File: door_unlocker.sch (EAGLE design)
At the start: 16 parts, among them IC1 LM2937, T1 2N3904

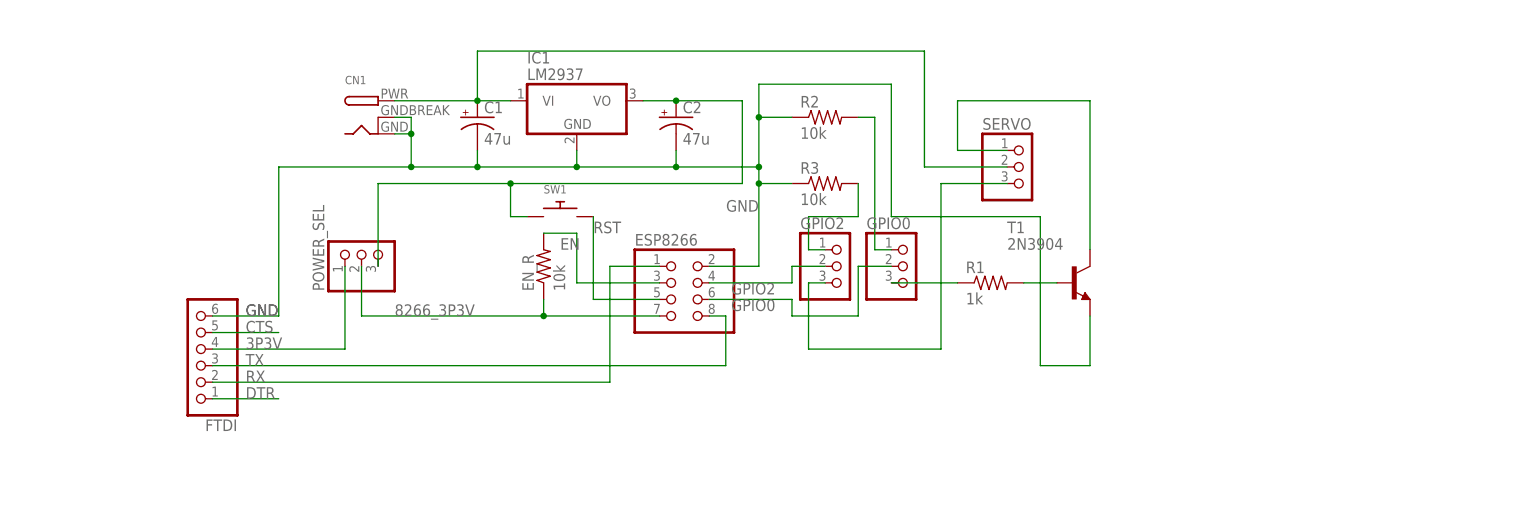
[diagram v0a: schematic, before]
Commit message: de-clusterfucked the schematic.
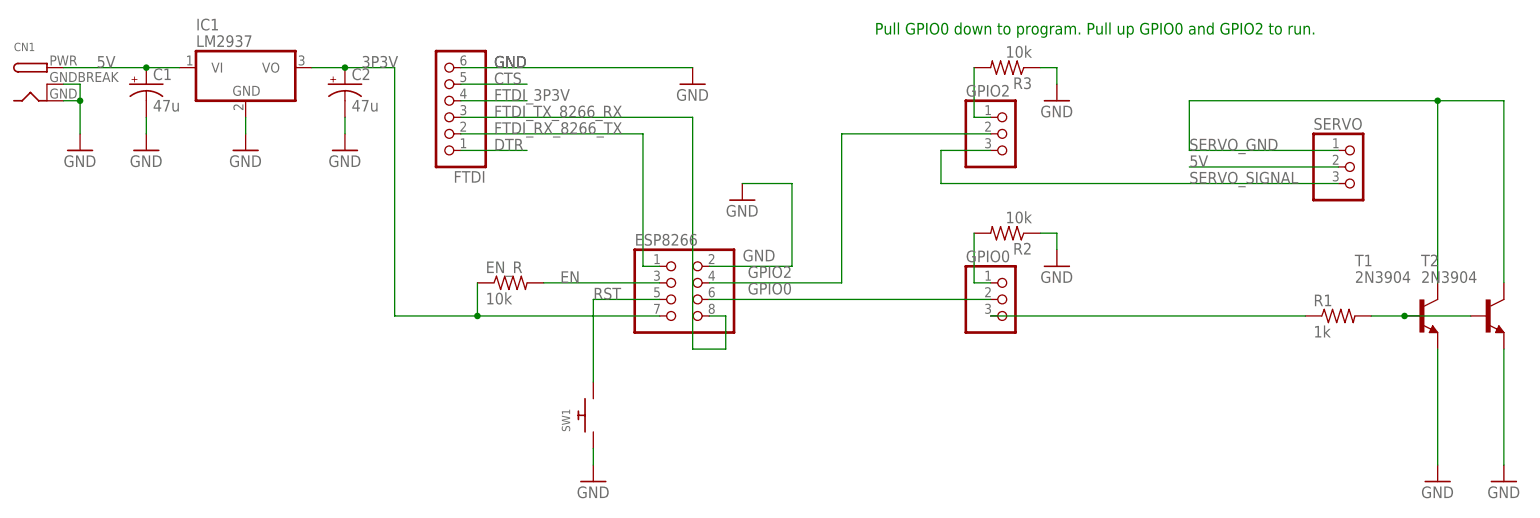
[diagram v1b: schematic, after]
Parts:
- removed POWER_SEL: (no value), adafruit:PINHD-1X3
- added T2: 2N3904, transistor:2N3904
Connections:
- net N$2 renamed 5V
- net N$9 renamed SERVO_SIGNAL
- net RX renamed FTDI_RX_8266_TX
- net TX renamed FTDI_TX_8266_RX
- removed net 8266_3P3V: EN_R.1, ESP8266.7, POWER_SEL.2
- removed net N$3: C2.+, IC1.VO, POWER_SEL.3, SW1.P$1
- removed net N$5: SERVO.1, T1.C
- new net FTDI_3P3V: FTDI.4
- new net SERVO_GND: SERVO.1, T1.C, T2.C
- net 3P3V: now also C2.+, EN_R.1, ESP8266.7, IC1.VO; no longer FTDI.4, POWER_SEL.1
- net GND: now also SW1.P$1, T2.E
- net N$8: now also T2.B
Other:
- note added: "Pull GPIO0 down to program. Pull up GPIO0 and GPIO2 to run."
- moved on the sheet: C1, C2, CN1, EN_R, FTDI, GPIO0, GPIO2, IC1, R1, R2, R3, SERVO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
